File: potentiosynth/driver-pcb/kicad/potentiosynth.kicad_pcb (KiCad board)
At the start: 2 copper layers, 127 x 63.5 mm, 71 parts, among them J1 Conn_01x40, U0 R-7815-0.5, U1 TLV9154IDR, U2 TLV9154IDR, U3 TLV9154IDR, U4 TLV9154IDR, U5 TLV9154IDR, U6 TLV9154IDR, U7 TLV9154IDR, U8 TLV9154IDR

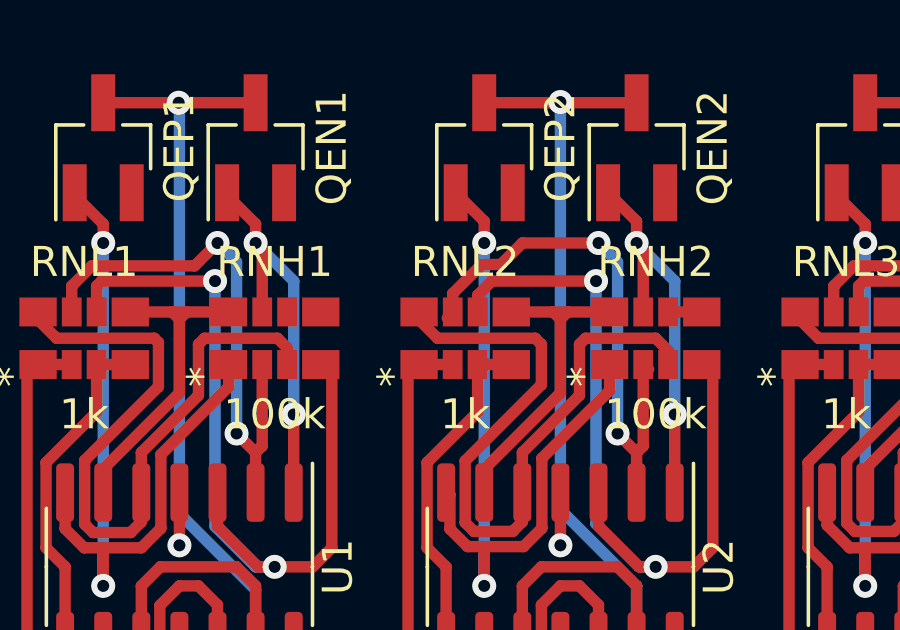
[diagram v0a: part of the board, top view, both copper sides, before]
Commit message: uncommitted changes
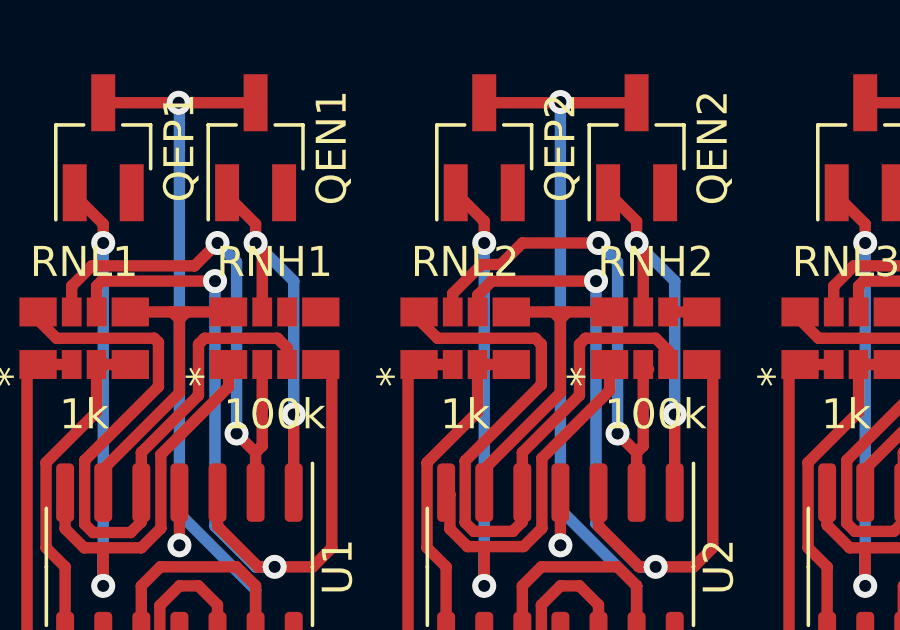
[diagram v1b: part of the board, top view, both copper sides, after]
